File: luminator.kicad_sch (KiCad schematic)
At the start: 4 parts

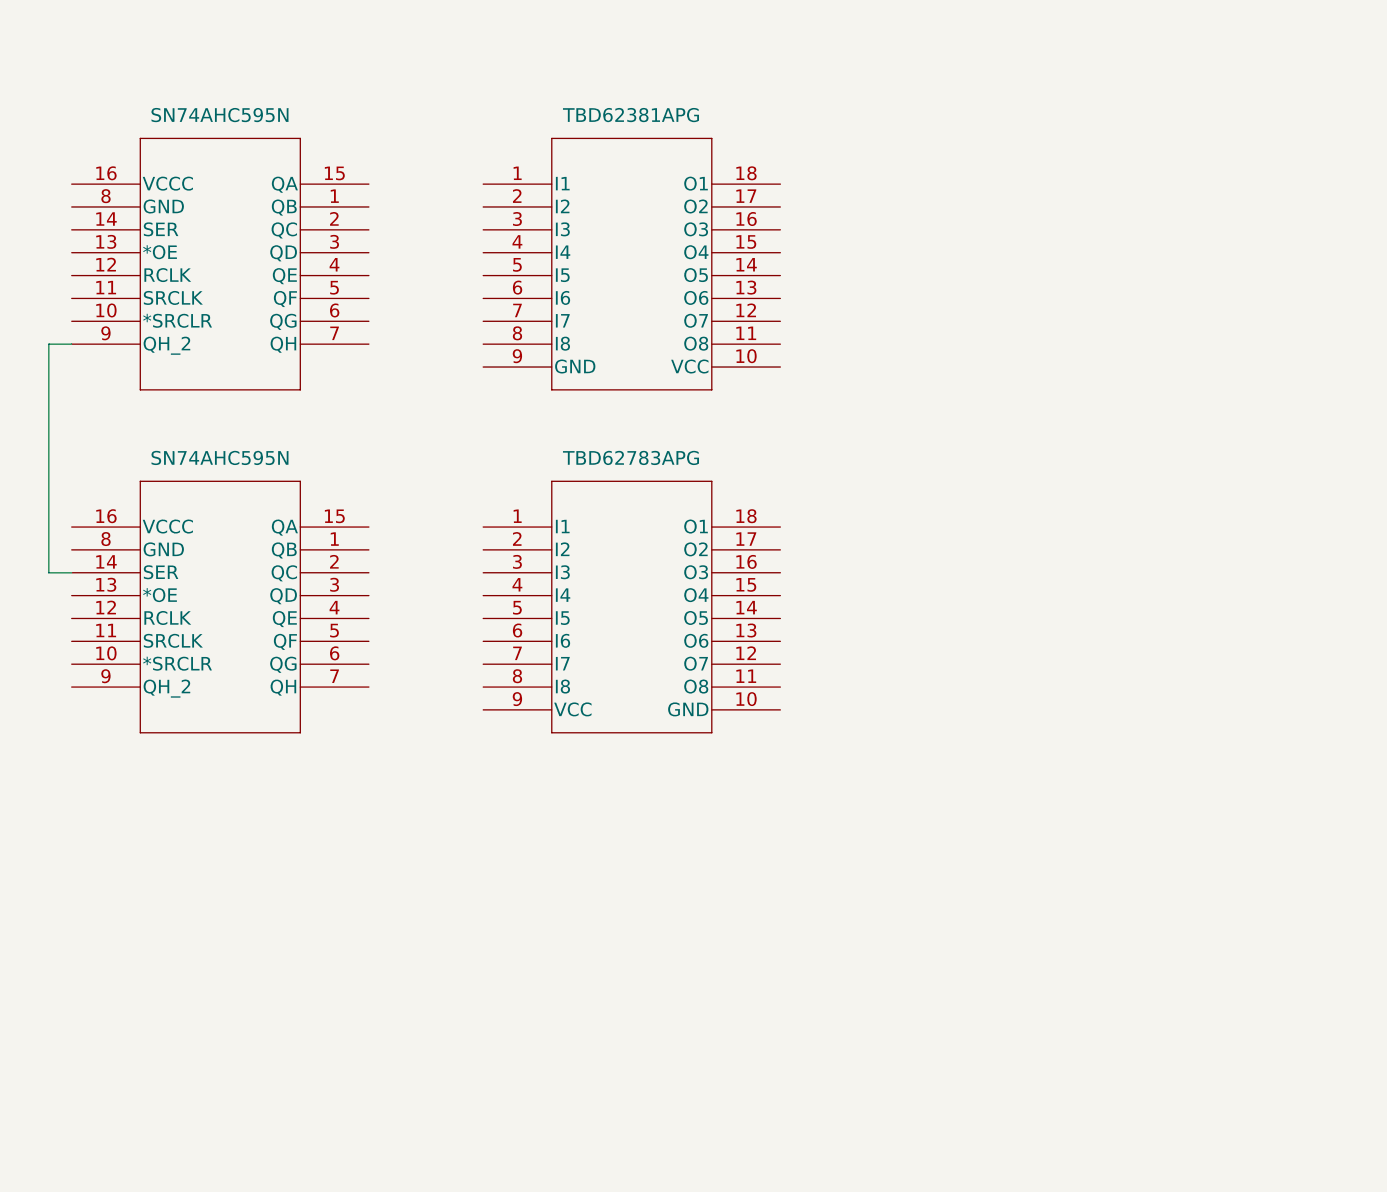
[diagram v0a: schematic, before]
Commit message: up
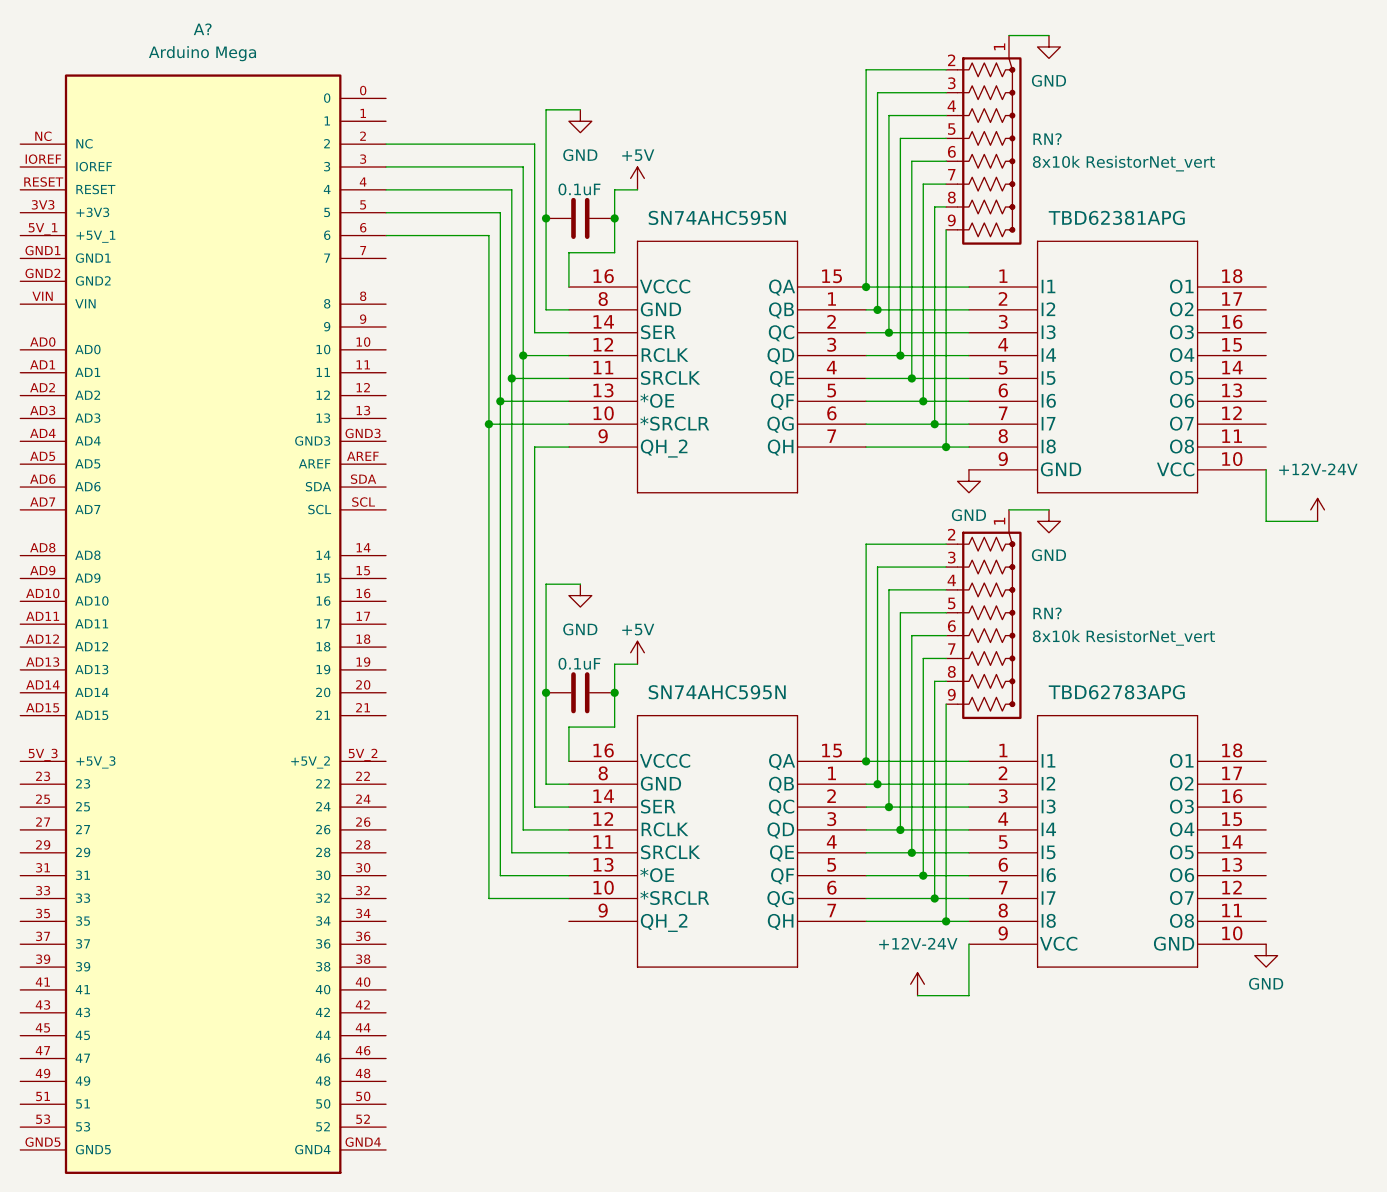
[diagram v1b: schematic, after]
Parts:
- added A?: Arduino Mega, ARDUINO_A000067, symbol Luminator:Arduino Mega
- added C? (x2): 0.1uF, symbol Device:C
- added RN? (x2): 8x10k ResistorNet_vert, Resistor_THT:R_Array_SIP10, symbol Luminator:8xResistorNet_vert
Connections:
- net at U?.1 (I1): now also U?.15 (QA), RN?.2 (R1) (x2)
- net GND: now reaches U?.10 (GND)
- net GND: now also U?.8 (GND), U?.8 (GND), U?.9 (GND), C?.1, C?.1, RN?.1 (common), RN?.1 (common)
- net at U?.2 (I2): now also U?.1 (QB), RN?.3 (R2) (x2)
- net at U?.3 (I3): now also U?.2 (QC), RN?.4 (R3) (x2)
- net at U?.4 (I4): now also U?.3 (QD), RN?.5 (R4) (x2)
- net at U?.5 (I5): now also U?.4 (QE), RN?.6 (R5) (x2)
- net at U?.6 (I6): now also U?.5 (QF), RN?.7 (R6) (x2)
- net at U?.7 (I7): now also U?.6 (QG), RN?.8 (R7) (x2)
- net at U?.8 (I8): now also U?.7 (QH), RN?.9 (R8) (x2)
- net +1V0: now reaches U?.9 (VCC)
- net +1V0: now also U?.10 (VCC)
- net at U?.10 (*SRCLR): now also U?.10 (*SRCLR), A?.6
- net at U?.11 (SRCLK): now also U?.11 (SRCLK), A?.4
- net at U?.12 (RCLK): now also U?.12 (RCLK), A?.3
- net at U?.13 (*OE): now also U?.13 (*OE), A?.5
- net +5V: now reaches U?.16 (VCCC)
- net +5V: now also U?.16 (VCCC), C?.2, C?.2
- net at U?.14 (SER): now also A?.2
